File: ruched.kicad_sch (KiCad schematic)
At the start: 23 parts, among them J20 USB_C_Receptacle_USB2.0 USB41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, Q6 UMH3N, Q7 DMG2301L, SW1 SW_Push, U1 CP2102N-A02-GQFN24

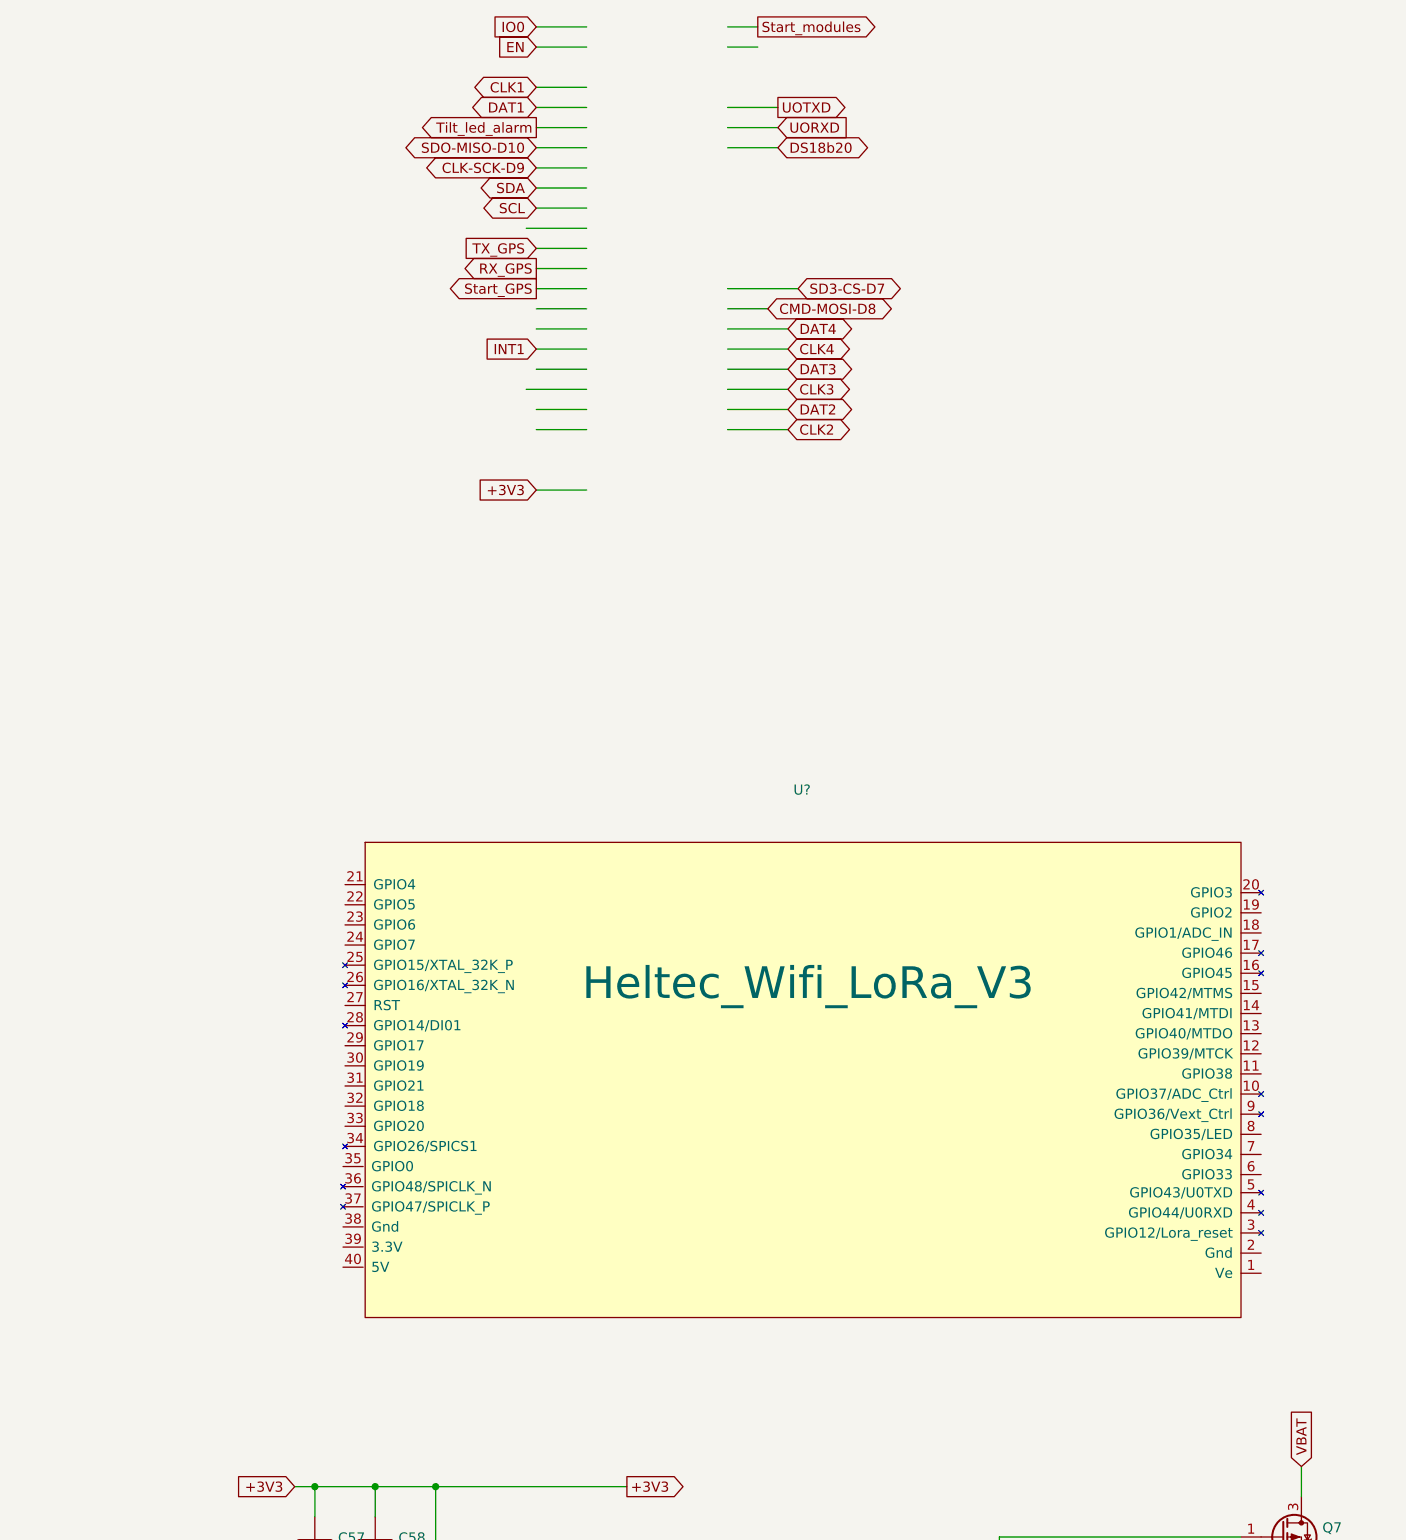
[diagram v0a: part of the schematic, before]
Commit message: Update
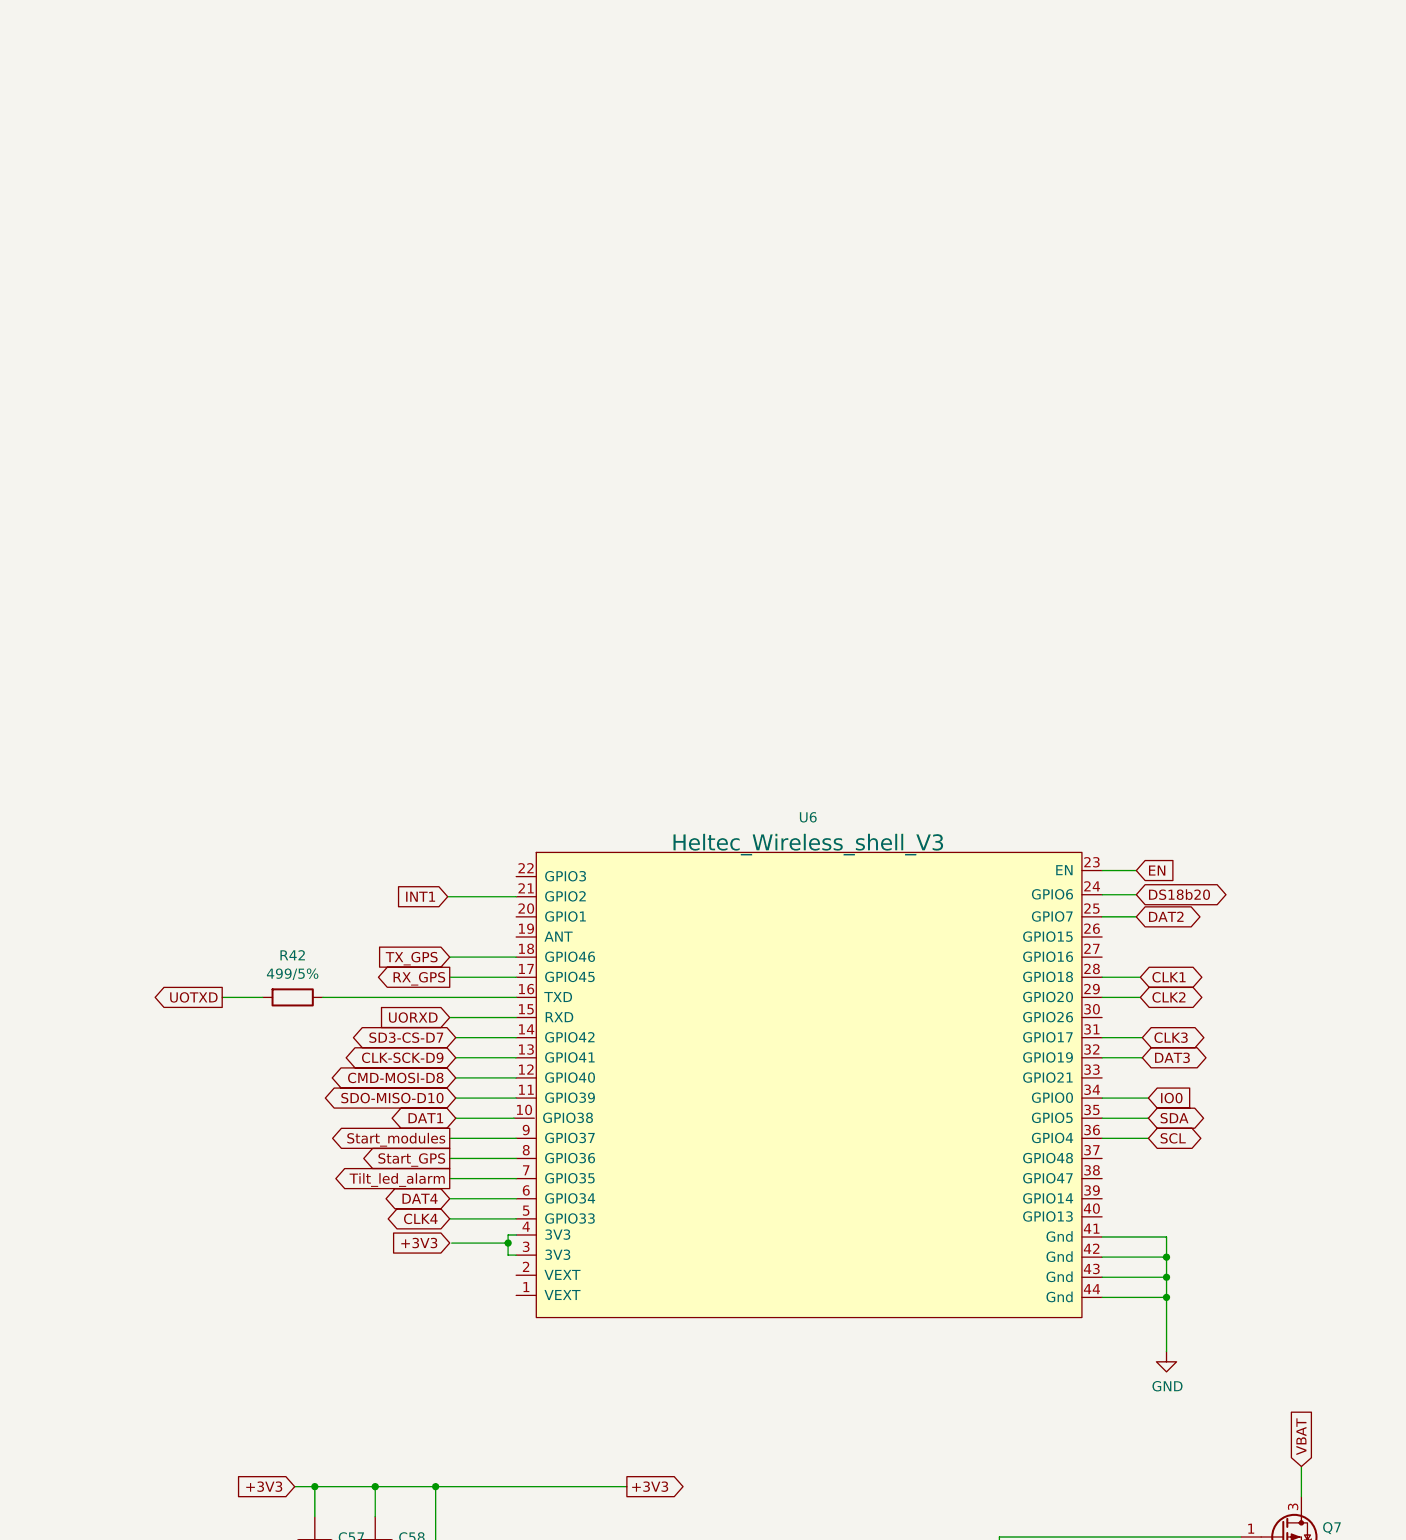
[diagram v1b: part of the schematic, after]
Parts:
- removed U?: Heltec_Wifi_LoRa_V3, symbol Espressif:Heltec_Wifi_LoRa_V3
- added R42: 499/5%, Resistor_SMD:R_0603_1608Metric, symbol Device:R
- added U6: Heltec_Wireless_shell_V3, Empreintes:Heltec Wireless shell V3, symbol Espressif:Heltec_Wireless_shell_V3
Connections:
- net CLK-SCK-D9: now also U6.13 (GPIO41)
- net CLK1: now also U6.28 (GPIO18)
- net CLK2: now also U6.29 (GPIO20)
- net CLK3: now also U6.31 (GPIO17)
- net CLK4: now also U6.5 (GPIO33)
- net CMD-MOSI-D8: now also U6.12 (GPIO40)
- net DAT1: now also U6.10 (GPIO38)
- net DAT2: now also U6.25 (GPIO7)
- net DAT3: now also U6.32 (GPIO19)
- net DAT4: now also U6.6 (GPIO34)
- net DS18b20: now also U6.24 (GPIO6)
- net EN: now also U6.23 (EN)
- net GND: now also U6.41 (Gnd), U6.42 (Gnd), U6.43 (Gnd), U6.44 (Gnd)
- net INT1: now also U6.21 (GPIO2)
- net IO0: now also U6.34 (GPIO0)
- net RX_GPS: now also U6.17 (GPIO45)
- net SCL: now also U6.36 (GPIO4)
- net SD3-CS-D7: now also U6.14 (GPIO42)
- net SDA: now also U6.35 (GPIO5)
- net SDO-MISO-D10: now also U6.11 (GPIO39)
- net Start_GPS: now also U6.8 (GPIO36)
- net Start_modules: now also U6.9 (GPIO37)
- net TX_GPS: now also U6.18 (GPIO46)
- net Tilt_led_alarm: now also U6.7 (GPIO35)
- net UORXD: now also U6.15 (RXD)
- net UOTXD: now also R42.2
- new net: R42.1, U6.16 (TXD)
- new net: U6.3 (3V3), U6.4 (3V3)

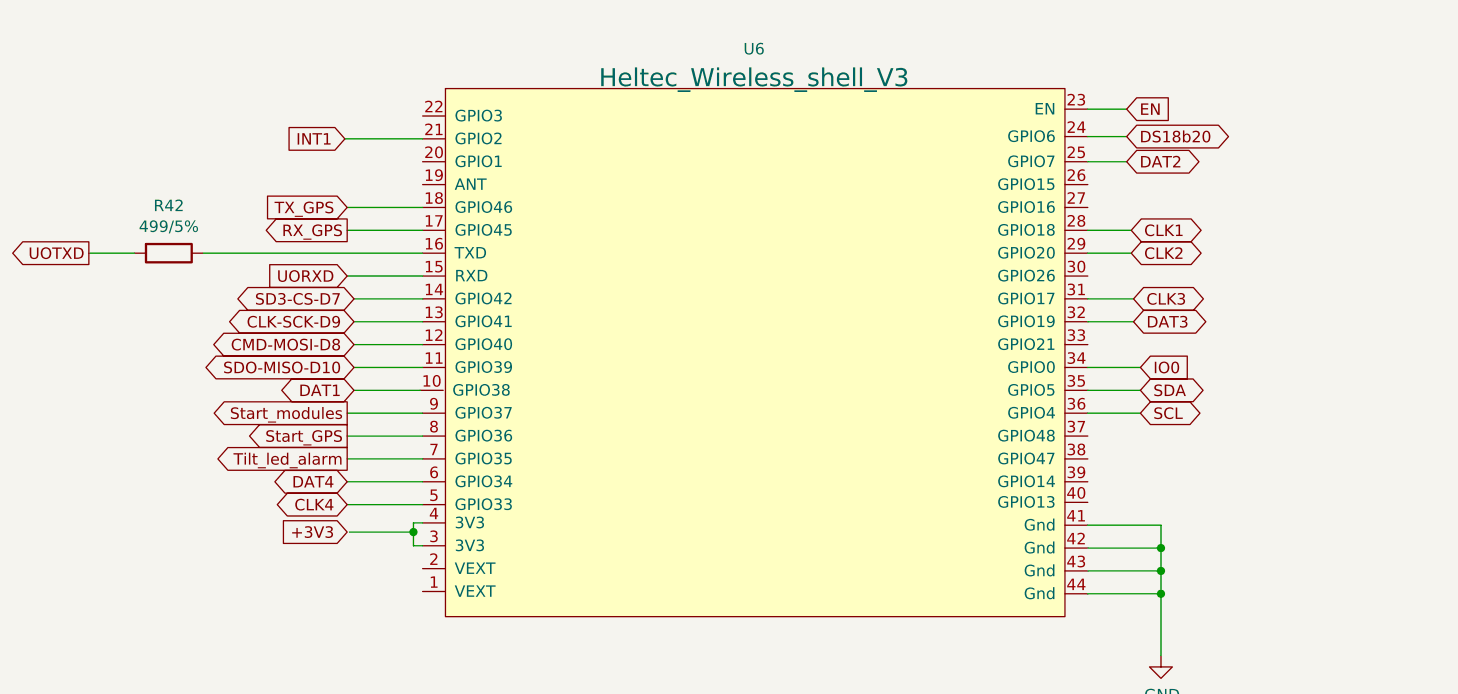
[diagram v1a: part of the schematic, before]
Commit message: Update
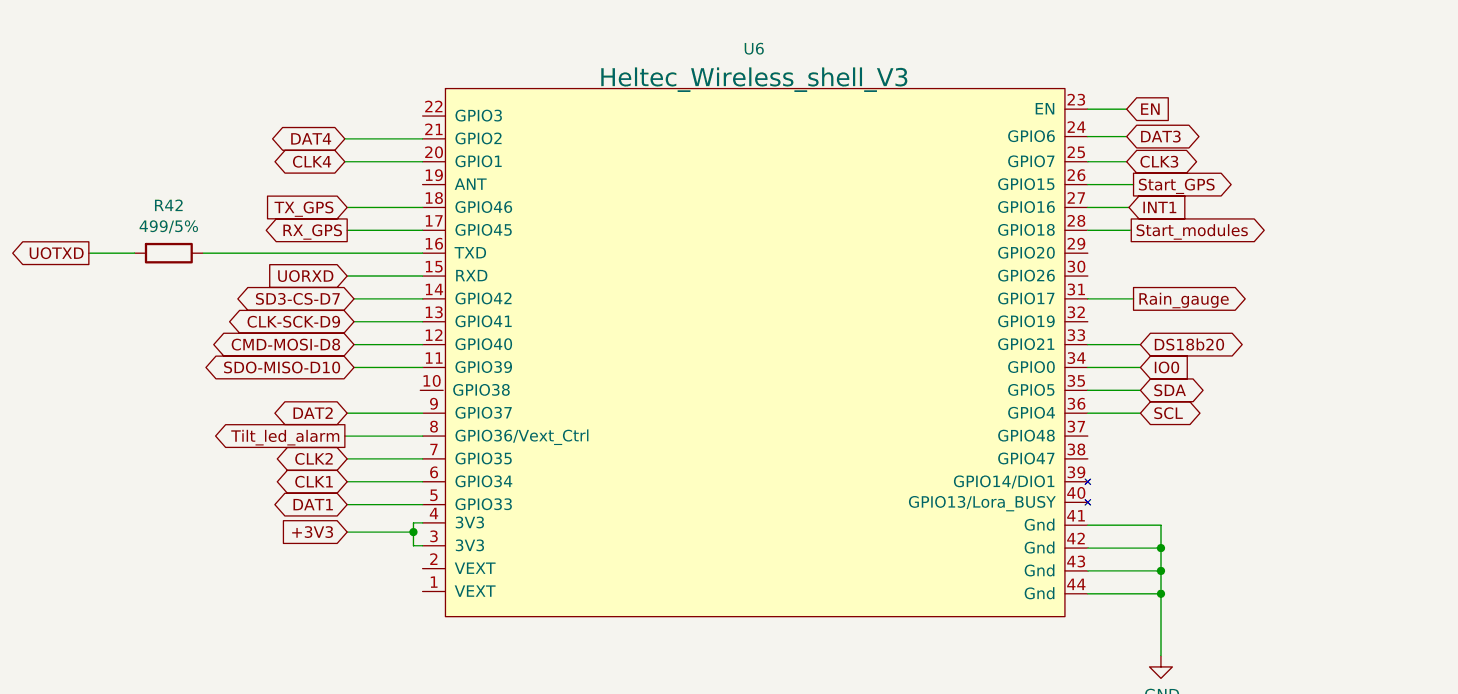
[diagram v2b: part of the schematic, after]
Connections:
- net +3V3: now also U6.3 (3V3), U6.4 (3V3)
- net CLK1: now also U6.6 (GPIO34); no longer U6.28 (GPIO18)
- net CLK2: now also U6.7 (GPIO35); no longer U6.29 (GPIO20)
- net CLK3: now also U6.25 (GPIO7); no longer U6.31 (GPIO17)
- net CLK4: now also U6.20 (GPIO1); no longer U6.5 (GPIO33)
- net DAT1: now also U6.5 (GPIO33); no longer U6.10 (GPIO38)
- net DAT2: now also U6.9 (GPIO37); no longer U6.25 (GPIO7)
- net DAT3: now also U6.24 (GPIO6); no longer U6.32 (GPIO19)
- net DAT4: now also U6.21 (GPIO2); no longer U6.6 (GPIO34)
- net DS18b20: now also U6.33 (GPIO21); no longer U6.24 (GPIO6)
- net INT1: now also U6.27 (GPIO16); no longer U6.21 (GPIO2)
- net Start_GPS: now also U6.26 (GPIO15); no longer U6.8 (GPIO36)
- net Start_modules: now also U6.28 (GPIO18); no longer U6.9 (GPIO37)
- net Tilt_led_alarm: now also U6.8 (GPIO36/Vext_Ctrl); no longer U6.7 (GPIO35)
- new net Rain_gauge: U6.31 (GPIO17)
